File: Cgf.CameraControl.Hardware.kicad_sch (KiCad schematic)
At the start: 28 parts, among them J1 5V input, J3 Pan, J4 Tilt, J5 SJ1-2503A, J6 Prog, J7 Sensor, Q2 BSS123, Q4 MUN5211DW1, Q5 BSS123, U1 WT32-ETH01, U2 DRV8212DRLR, U3 TXS0102DCT, U4 DRV8212DRLR, U5 TXS0101DCK

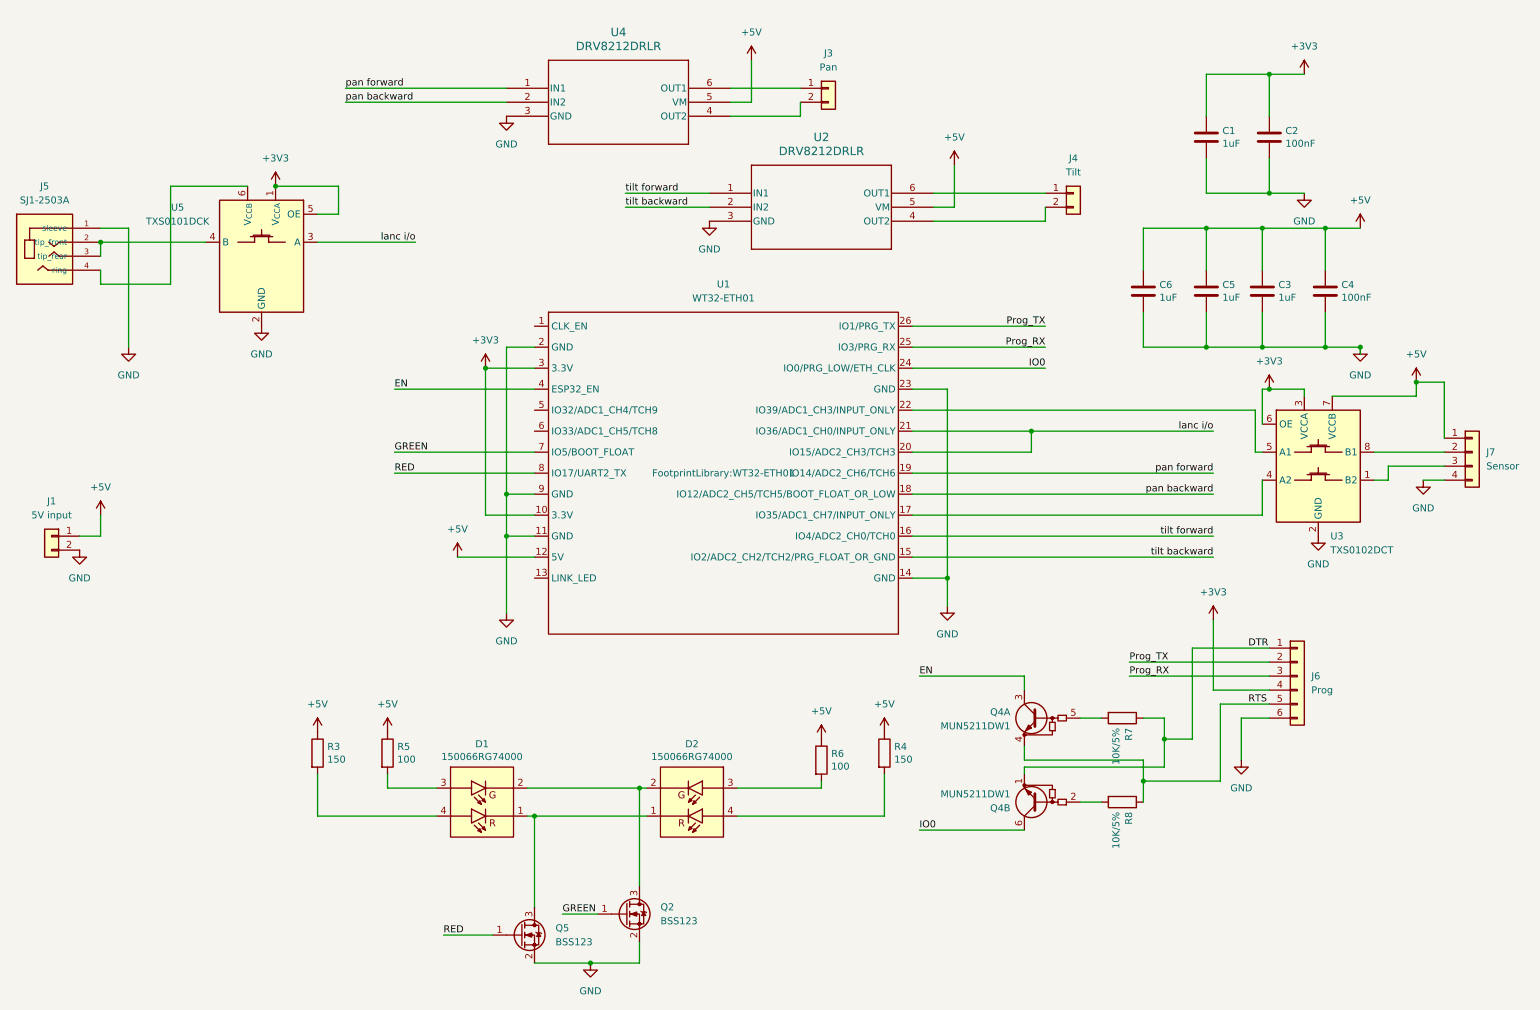
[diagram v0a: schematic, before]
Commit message: Apply suggestions from review
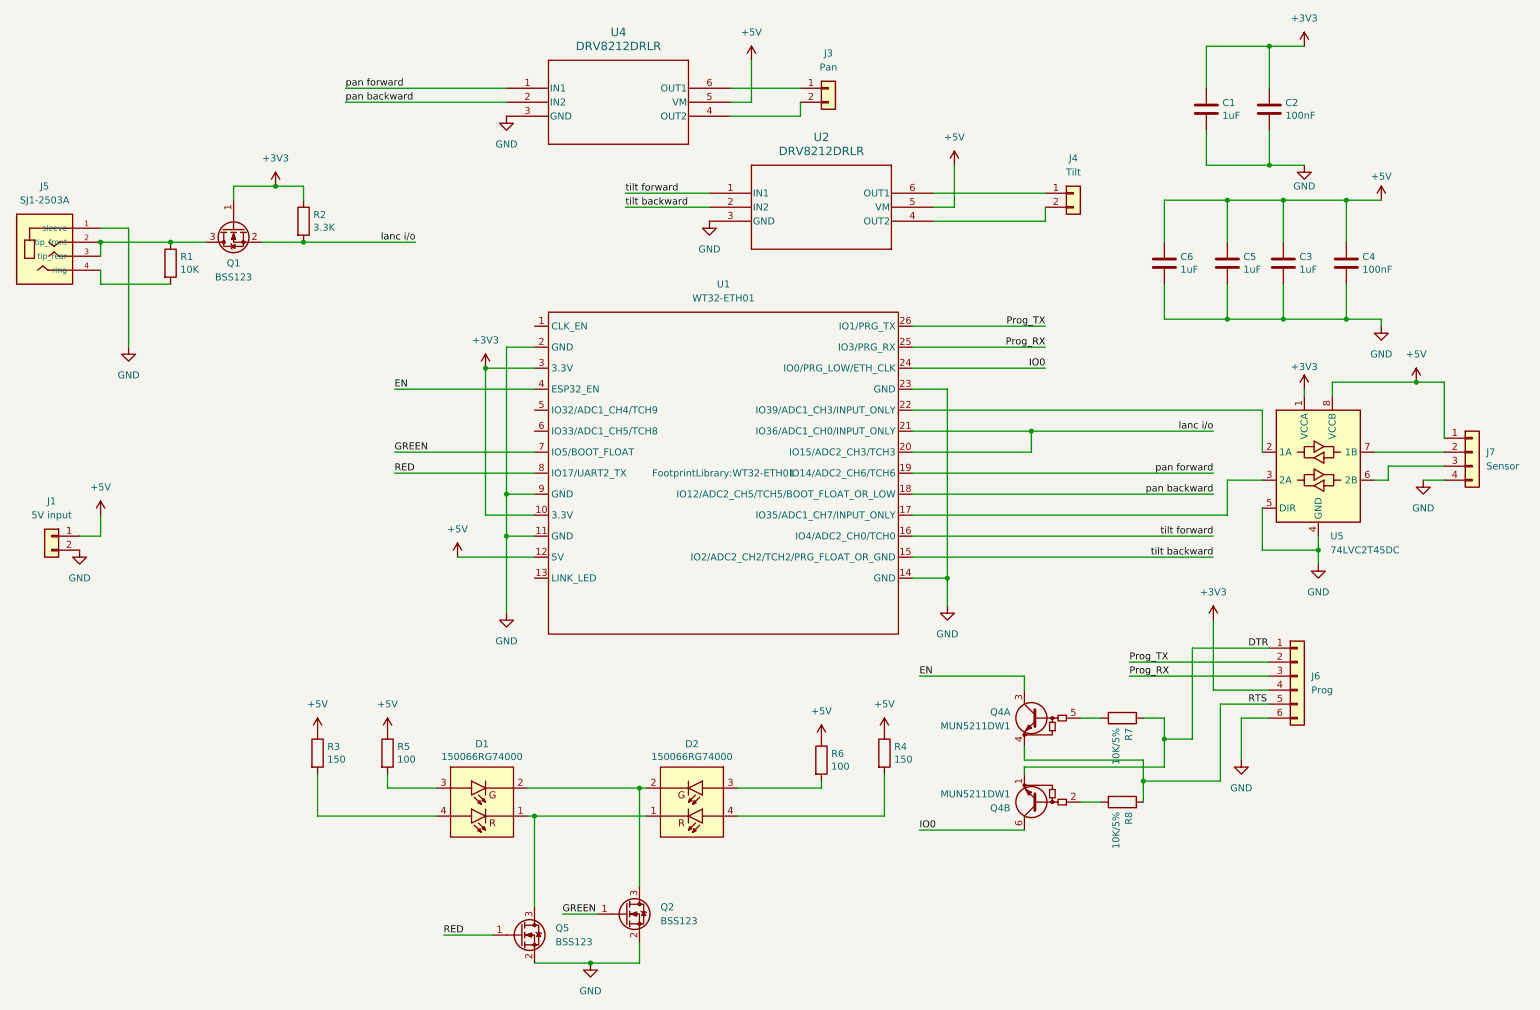
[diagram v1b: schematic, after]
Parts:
- removed U3: TXS0102DCT, Package_SO:SSOP-8_2.95x2.8mm_P0.65mm, symbol Logic_LevelTranslator:TXS0102DCT
- removed U5: TXS0101DCK, Package_TO_SOT_SMD:SOT-363_SC-70-6, symbol Logic_LevelTranslator:TXS0101DCK
- added Q1: BSS123, Package_TO_SOT_SMD:SOT-23, symbol Transistor_FET:BSS123
- added R1: 10K, Resistor_SMD:R_0805_2012Metric, symbol Device:R
- added R2: 3.3K, Resistor_SMD:R_0805_2012Metric, symbol Device:R
- added U5: 74LVC2T45DC, Package_SO:VSSOP-8_2.3x2mm_P0.5mm, symbol Logic_LevelTranslator:74LVC2T45DC
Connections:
- net +3V3: now also Q1.1 (G), R2.1, U5.1 (VCCA)
- net +5V: now also U5.8 (VCCB)
- net GND: now also U5.4 (GND), U5.5 (DIR)
- net lanc i/o: now also Q1.2 (S), R2.2
- net at J5.2 (tip_front), J5.3 (tip_rear): now also Q1.3 (D), R1.1
- net at J5.4 (ring): now also R1.2
- net at U1.17 (IO35/ADC1_CH7/INPUT_ONLY): now also U5.3 (2A)
- net at U1.22 (IO39/ADC1_CH3/INPUT_ONLY): now also U5.2 (1A)
- net at J7.2 (Pin_2): now also U5.7 (1B)
- net at J7.3 (Pin_3): now also U5.6 (2B)
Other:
- moved on the sheet: C1, C2, C3, C4, C5, C6
